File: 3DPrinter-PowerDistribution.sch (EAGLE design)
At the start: 30 parts, among them J1 Extruder 1, J2 24V Input, J3 To Motor Drivers, J4 To microcontroller board, J5 Extruder 2, J6 Bed Heater, Q1 PSMN1R3-30YL, Q2 PSMN1R3-30YL, Q3 PSMN1R3-30YL, Q4 PSMN1R3-30YL, Q5 PSMN1R3-30YL, Q6 PSMN1R3-30YL

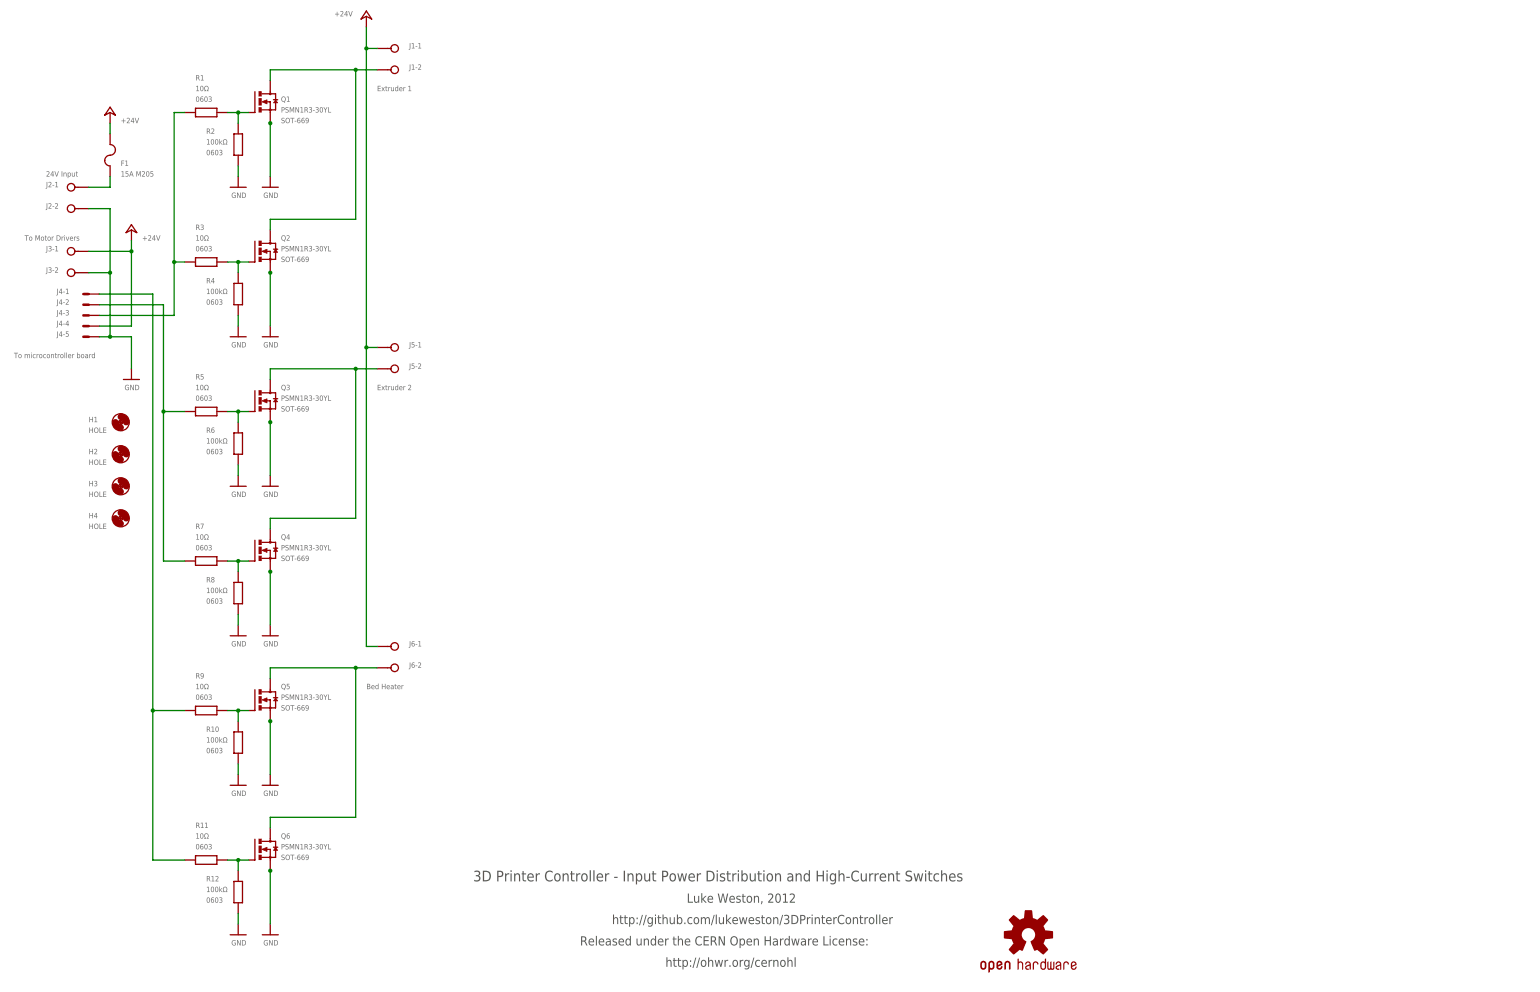
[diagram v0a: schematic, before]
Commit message: foo
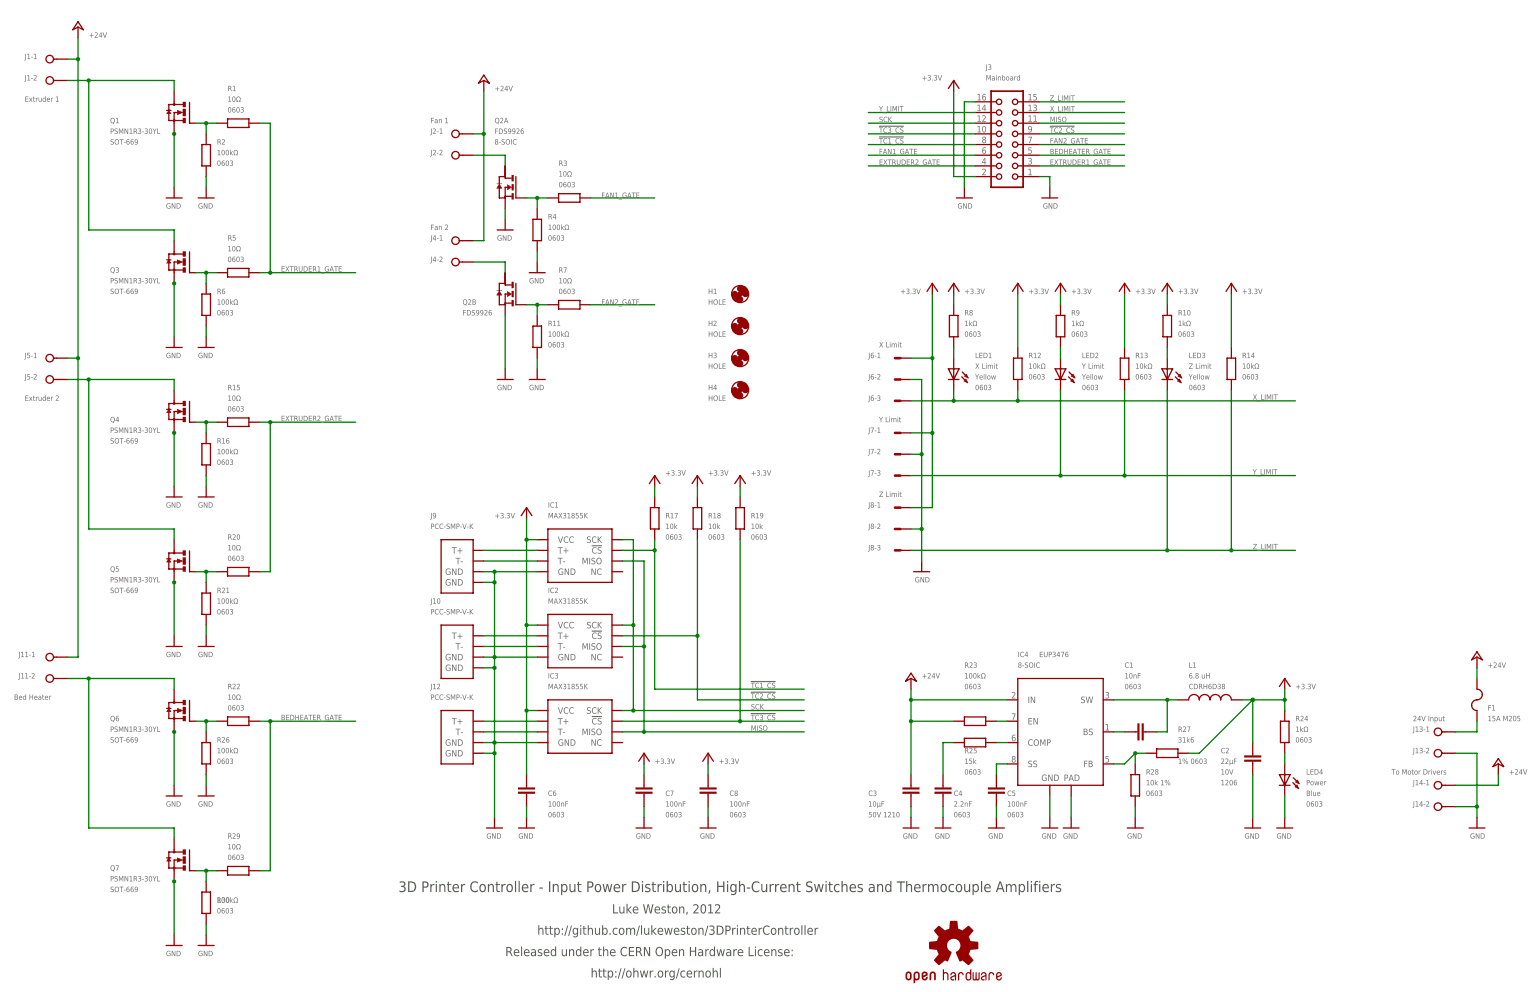
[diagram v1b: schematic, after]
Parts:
- removed SY5: OSHW-LOGOS, SparkFun:OSHW-LOGOS
- added C1: 10nF, freetronics-master-v1:CAP0603
- added C2: 22µF, freetronics-jon:C-EUC1206K
- added C3: 10µF, freetronics-jon:C-EUC1210K
- added C4: 2.2nF, freetronics-master-v1:CAP0603
- added C5, C6, C7, C8: 100nF, freetronics-master-v1:CAP0603
- added IC1, IC2, IC3: MAX31855K, RAMPSdisplay:MCLENG_MAX6675MAX31855
- added IC4: EUP3476, freetronics-luke:EUP3476
- added J10, J12, J9: PCC-SMP-V-K, RAMPSdisplay:MCLAUGHLINENG_TC_JACK
- added J11: Bed Heater, con-wago-508:W237-02P
- added J13: 24V Input, con-wago-508:W237-02P
- added J14: To Motor Drivers, con-wago-508:W237-02P
- added J7: Y Limit, con-molex:22-05-7038-03
- added J8: Z Limit, con-molex:22-05-7038-03
- added L1: 6.8 uH, freetronics-luke:INDUCTOR
- added LED1: X Limit, freetronics-master-v1:LED0603
- added LED2: Y Limit, freetronics-master-v1:LED0603
- added LED3: Z Limit, freetronics-master-v1:LED0603
- added LED4: Power, freetronics-master-v1:LED0603
- added Q7: PSMN1R3-30YL, transistor-power:PH7030L
- added R13, R14: 10kΩ, freetronics-master-v1:RESISTOR0603
- added R15, R20, R22, R29: 10Ω, freetronics-master-v1:RESISTOR0603
- added R16, R21, R23, R26, R30: 100kΩ, freetronics-master-v1:RESISTOR0603
- added R17, R18, R19: 10k, freetronics-master-v1:RESISTOR0603
- added R24: 1kΩ, freetronics-master-v1:RESISTOR0603
- added R25: 15k, freetronics-master-v1:RESISTOR0603
- added R27: 31k6, freetronics-master-v1:RESISTOR0603
- added R28: 10k 1%, freetronics-master-v1:RESISTOR0603
- added SY: OSHW-LOGOS, SparkFun:OSHW-LOGOS
- J2: value 24V Input -> Fan 1; OC_FARNELL (none) -> unknown; OC_NEWARK (none) -> unknown
- J3: value To Motor Drivers -> Mainboard; device con-wago-508:W237-02P -> con-harting:CON16L
- J4: value To microcontroller board -> Fan 2; device con-molex:22-23-2051 -> con-wago-508:W237-02P; OC_FARNELL (none) -> unknown; OC_NEWARK (none) -> unknown
- J6: value Bed Heater -> X Limit; device con-wago-508:W237-02P -> con-molex:22-05-7038-03
- Q2: value PSMN1R3-30YL -> FDS9926; device transistor-power:PH7030L -> zetex:NMOS2SM8; OC_FARNELL (none) -> unknown; OC_NEWARK (none) -> unknown; PACKAGE SOT-669 -> 8-SOIC
- R10, R8: value 100kΩ -> 1kΩ
- R11: value 10Ω -> 100kΩ
- R12: value 100kΩ -> 10kΩ
- R9: value 10Ω -> 1kΩ
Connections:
- removed net N$1 (its old number): Q2.G, R3.2, R4.1
- new net !TC1_CS: IC1.!CS, J3.8, R17.2
- new net !TC2_CS: IC2.!CS, J3.9, R18.2
- new net !TC3_CS: IC3.!CS, J3.10, R19.2
- new net +3.3V: C2.1, C6.1, C7.1, C8.1, IC1.VCC, IC2.VCC, IC3.VCC, J3.2, J6-1.S, J7-1.S, J8-1.S, L1.2, R10.1, R12.1, R13.1, R14.1, R17.1, R18.1, R19.1, R24.1, R27.1, R8.1, R9.1
- new net BEDHEATER_GATE: J3.5, R22.1, R29.1
- new net EXTRUDER1_GATE: J3.3, R1.1, R5.1
- new net EXTRUDER2_GATE: J3.4, R15.1, R20.1
- new net FAN1_GATE: J3.6, R3.1
- new net FAN2_GATE: J3.7, R7.1
- new net MISO: IC1.MISO, IC2.MISO, IC3.MISO, J3.11
- new net N$10: J2-2.KL, Q2A.D
- new net N$12: J4-2.KL, Q2B.D
- new net N$13: Q2A.G, R3.2, R4.1
- new net N$15: LED1.A, R8.2
- new net N$16: LED2.A, R9.2
- new net N$17: LED3.A, R10.2
- new net N$21: LED4.A, R24.2
- new net N$28: IC3.T-, J12.T-
- new net N$29: IC3.T+, J12.T+
- new net N$3: Q4.G, R15.2, R16.1
- new net N$32: IC2.T-, J10.T-
- new net N$33: IC2.T+, J10.T+
- new net N$42: IC4.EN, R23.1
- new net N$44: C1.1, IC4.SW, L1.1
- new net N$51: C1.2, IC4.BS
- new net N$59: C4.2, R25.2
- new net N$61: IC4.COMP, R25.1
- new net N$62: C5.2, IC4.SS
- new net N$63: IC4.FB, R27.2, R28.1
- new net SCK: IC1.SCK, IC2.SCK, IC3.SCK, J3.12
- new net X_LIMIT: J3.13, J6-3.S, LED1.C, R12.2
- new net Y_LIMIT: J3.14, J7-3.S, LED2.C, R13.2
- new net Z_LIMIT: J3.15, J8-3.S, LED3.C, R14.2
- net +24V: now also C3.1, IC4.IN, J11-1.KL, J14-1.KL, J2-1.KL, J4-1.KL, R23.2; no longer J3-1.KL, J4-4.S, J6-1.KL
- net GND: now also C2.2, C3.2, C4.1, C5.1, C6.2, C7.2, C8.2, IC1.GND, IC2.GND, IC3.GND, IC4.GND, IC4.TGND, J10.GND, J10.GND@1, J12.GND, J12.GND@1, J13-2.KL, J14-2.KL, J3.1, J3.16, J6-2.S, J7-2.S, J8-2.S, J9.GND, J9.GND@1, LED4.C, Q2A.S, Q2B.S, Q7.S, Q7.S@1, Q7.S@2, R11.2, R16.2, R21.2, R26.2, R28.2, R30.2; no longer J2-2.KL, J3-2.KL, J4-5.S, Q2.S, Q2.S@1, Q2.S@2, R10.2, R12.2, R8.2
- net J5: now also J11-2.KL, Q7.D; no longer J6-2.KL, Q5.D
- net N$11: now also IC1.T-, J9.T-; no longer J4-2.S, R5.1, R7.1
- net N$14: now also Q2B.G, R11.1, R7.2; no longer J4-3.S, R1.1, R3.1
- net N$2: now also Q3.D; no longer Q2.D
- net N$4: now also Q5.D; no longer Q3.D
- net N$5: now also Q5.G, R20.2, R21.1; no longer Q4.G, R7.2, R8.1
- net N$6: now also J13-1.KL; no longer J2-1.KL
- net N$7: now also Q6.G, R22.2, R26.1; no longer Q5.G, R10.1, R9.2
- net N$8: now also IC1.T+, J9.T+; no longer J4-1.S, R11.1, R9.1
- net N$9: now also Q7.G, R29.2, R30.1; no longer Q6.G, R11.2, R12.1
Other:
- note added: "2x Lower-current Outputs"
- note added: "3 x Limit Switches"
- note added: "3.3V Buck Regulator (EUP3476)"
- note added: "3D Printer Controller - Input Power Distribution, High-Current Switches and Thermocouple Amplifiers"
- note added: "3x 24V High-Current Open-Drain Outputs"
- note added: "3x K-type Thermocouples (MAX31855Ks)"
- note added: "For driving fans, etc."
- note added: "The recommended limit sensors are Diodes Inc. AH180 omnipolar Hall effect switches (Digi-Key AH180-PL-ADICT-ND). Note that Hall effect sensors with an analog voltage output are not the same and cannot be used. Conventional normally-open switches may also be used, but optical slot interrupters are not supported as there are no connections for power to the infrared LEDs."
- note added: "Thermocouple connectors are Omega PCC-SMP-V-K minature vertical PCB-mount. Change MAX31855x thermocouple type and Omega PCC-SMP-V-x metallurgy type if the thermocouple type is not K-type."
- note removed: "3D Printer Controller - Input Power Distribution and High-Current Switches"
- moved on the sheet: F1, H1, H2, H3, H4, J1-1, J1-2, J2-1, J2-2, J5-1, J5-2, Q1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
